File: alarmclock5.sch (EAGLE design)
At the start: 44 parts, among them Q1 FDN360P, T1 2N2222, X1 MKDSN1,5/2-5,08, X2 MKDSN1,5/2-5,08, X3 MKDSN1,5/2-5,08, X4 MKDSN1,5/2-5,08

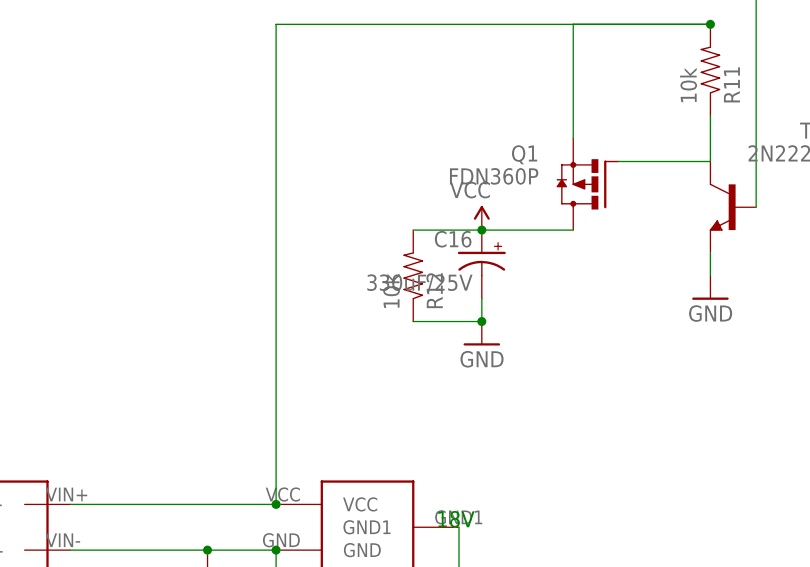
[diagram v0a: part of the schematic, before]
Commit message: update especially mouser.lbr
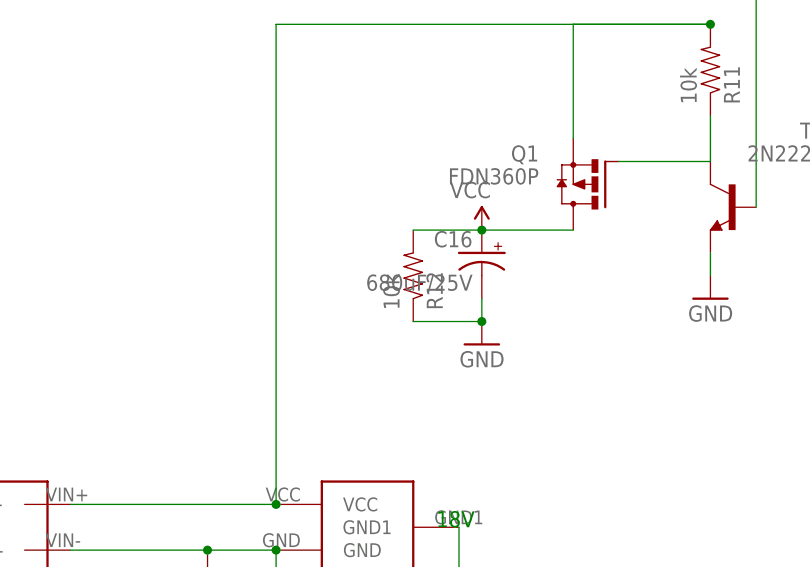
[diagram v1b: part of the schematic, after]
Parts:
- C16: value 330uF/25V -> 680uF/25V
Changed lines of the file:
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@@
 <part name="GND3" library="SparkFun-Aesthetics" deviceset="GND" device=""/>
 <part name="SUPPLY31" library="SparkFun-Aesthetics" deviceset="VCC" device=""/>
-<part name="C16" library="SparkFun-Passives" deviceset="CAP_POL" device="PTH2" value="330uF/25V"/>
+<part name="C16" library="SparkFun-Passives" deviceset="CAP_POL" device="PTH2" value="680uF/25V"/>
 <part name="R12" library="SparkFun-Passives" deviceset="RESISTOR" device="0603-RES" value="10k"/>
 </parts>
